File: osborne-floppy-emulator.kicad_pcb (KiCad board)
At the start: 2 copper layers, 76.2 x 94 mm, 67 parts, among them J1 Connector Out, J2 USB_A, J3 SWD Connector, J4 Connector In, Q1 BC557, Q2 BC547, Q3 T2N7002BK, Q4 BC547, Q5 BC547, Q6 BC547, Q7 BC547, Q8 BC547, Q9 BC547, U1 W25Q16JVSSIM, U2 RP2040, U3 TL494

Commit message: fixed issue with OCP comparator polarity
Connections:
- R13 pad 2: Net-(U3-2IN+) -> Net-(U3-2IN-)
- R9 pad 1: Net-(U3-2IN+) -> Net-(U3-2IN-)
- U3 pad 15: GND -> Net-(U3-2IN-)
- U3 pad 16: Net-(U3-2IN+) -> GND
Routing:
- net Net-(U3-2IN-): track 0.00 -> 66.5 mm
- net GND: track 107.9 -> 41.4 mm
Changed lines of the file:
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@@
 	(net 59 "Net-(R12-Pad1)")
 	(net 60 "Net-(U3-1IN+)")
-	(net 61 "Net-(U3-2IN+)")
+	(net 61 "Net-(U3-2IN-)")
 	(net 62 "Net-(U3-RT)")
 	(net 63 "/Processor/Chip D+")
@@
 			)
 		)
-		(property "Mouser part no." " 603-MFR-25FTE52-7K5"
+		(property "Mouser part no." " 603-MFR-12FTF52-7K5"
 			(at 0 0 30)
 			(unlocked yes)
@@
 			)
 		)
-		(property "Mouser part no." " 603-MFR-25FTE52-27K"
+		(property "Mouser part no." " 603-MFR-12FTF52-27K"
 			(at 0 0 -135)
 			(unlocked yes)
@@
 			)
 		)
-		(property "Mouser part no." " 603-MFR-25FTE52-3K6 "
+		(property "Mouser part no." " 603-MFR-12FTF52-3K6 "
 			(at 0 0 -75)
 			(unlocked yes)
@@
 			)
 		)
-		(property "Mouser part no." " 603-MFR-25FTE52-27K"
+		(property "Mouser part no." " 603-MFR-12FTF52-27K"
 			(at 0 0 -120)
 			(unlocked yes)
@@
 			)
 		)
-		(property "Mouser part no." " 737-PH2-18-UA"
+		(property "Mouser part no." " 649-67996-434HLF"
 			(at 0 0 0)
 			(unlocked yes)
@@
 			)
 		)
-		(property "Mouser part no." " 603-MFR-25FTE52-27K"
+		(property "Mouser part no." " 603-MFR-12FTF52-27K"
 			(at 0 0 180)
 			(unlocked yes)
@@
 			)
 		)
-		(property "Mouser part no." " 603-MFR-25FTE52-27K"
+		(property "Mouser part no." " 603-MFR-12FTF52-27K"
 			(at 0 0 0)
 			(unlocked yes)
@@
 			(layers "*.Cu" "*.Mask")
 			(remove_unused_layers no)
-			(net 5 "GND")
+			(net 61 "Net-(U3-2IN-)")
 			(pinfunction "2IN-")
 			(pintype "input")
@@
 			(layers "*.Cu" "*.Mask")
 			(remove_unused_layers no)
-			(net 61 "Net-(U3-2IN+)")
+			(net 5 "GND")
 			(pinfunction "2IN+")
 			(pintype "input")
@@
 			)
 		)
-		(property "Mouser part no." " 737-RS2-20-G"
+		(property "Mouser part no." " 710-61304021821"
 			(at 0 0 180)
 			(unlocked yes)
@@
 			)
 		)
-		(property "Mouser part no." " 603-MFR-25FTE52-56R"
+		(property "Mouser part no." " 603-MFR-12FTF52-56R"
 			(at 0 0 180)
 			(unlocked yes)
@@
 			(layers "*.Cu" "*.Mask")
 			(remove_unused_layers no)
-			(net 61 "Net-(U3-2IN+)")
+			(net 61 "Net-(U3-2IN-)")
 			(pintype "passive")
 		)
@@
 			)
 		)
-		(property "Mouser part no." " 603-MFR-25FTE52-27K"
+		(property "Mouser part no." " 603-MFR-12FTF52-27K"
 			(at 0 0 165)
 			(unlocked yes)
@@
 			)
 		)
-		(property "Mouser part no." " 603-MFR-25FTE52-27K"
+		(property "Mouser part no." " 603-MFR-12FTF52-27K"
 			(at 0 0 165)
 			(unlocked yes)
@@
 			)
 		)
-		(property "Mouser part no." " 603-MFR-25FTE52-27K"
+		(property "Mouser part no." " 603-MFR-12FTF52-27K"
 			(at 0 0 180)
 			(unlocked yes)
@@
 			)
 		)
-		(property "Mouser part no." " 603-MFR-25FTE52-12K"
+		(property "Mouser part no." " 603-MFR-12FTF52-12K"
 			(at 0 0 150)
 			(unlocked yes)
@@
 			)
 		)
-		(property "Mouser part no." " 603-MFR-25FTE52-27K"
+		(property "Mouser part no." " 603-MFR-12FTF52-27K"
 			(at 0 0 150)
 			(unlocked yes)
@@
 			)
 		)
-		(property "Mouser part no." " 603-MFR-25FTE52-27K"
+		(property "Mouser part no." " 603-MFR-12FTF52-27K"
 			(at 0 0 180)
 			(unlocked yes)
@@
 			)
 		)
-		(property "Mouser part no." " 603-MFR-25FTE52-27K"
+		(property "Mouser part no." " 603-MFR-12FTF52-27K"
 			(at 0 0 90)
 			(unlocked yes)
@@
 			(layers "*.Cu" "*.Mask")
 			(remove_unused_layers no)
-			(net 61 "Net-(U3-2IN+)")
+			(net 61 "Net-(U3-2IN-)")
 			(pintype "passive")
 		)
@@
 	)
 	(segment
-		(start 153.6 38.8)
-		(end 155 37.2)
-		(width 0.6)
-		(layer "F.Cu")
-		(net 5)
-	)
-	(segment
 		(start 150.2 85.6)
 		(end 149.2 86.2)
@@
 	)
 	(segment
-		(start 155.4 34.8)
-		(end 155.4 25)
-		(width 0.6)
-		(layer "F.Cu")
-		(net 5)
-	)
-	(segment
 		(start 151.8 88.0625)
 		(end 151.2 89.6)
@@
 	)
 	(segment
-		(start 151.599999 39.000001)
-		(end 153.6 38.8)
-		(width 0.6)
-		(layer "F.Cu")
-		(net 5)
-	)
-	(segment
-		(start 155.4 25)
-		(end 153.6 19.6)
-		(width 0.6)
-		(layer "F.Cu")
-		(net 5)
-	)
-	(segment
 		(start 143.2 91.6)
 		(end 142.4 92.8)
@@
 	)
 	(segment
-		(start 148.2 16.4)
-		(end 112.6 16.4)
-		(width 0.6)
-		(layer "F.Cu")
-		(net 5)
-	)
-	(segment
 		(start 124.700001 40.599999)
 		(end 124.6 43)
@@
 	)
 	(segment
-		(start 149.02 38.96)
-		(end 151.599999 39.000001)
-		(width 0.6)
-		(layer "F.Cu")
-		(net 5)
-	)
-	(segment
 		(start 116.6 38.499999)
 		(end 118.2 35.2)
@@
 	)
 	(segment
-		(start 153.6 19.6)
-		(end 148.2 16.4)
-		(width 0.6)
-		(layer "F.Cu")
-		(net 5)
-	)
-	(segment
 		(start 151.2 85)
 		(end 150.2 85.6)
@@
 	)
 	(segment
-		(start 155 37.2)
-		(end 155.4 34.8)
-		(width 0.6)
-		(layer "F.Cu")
-		(net 5)
-	)
-	(segment
 		(start 159.466222 82.046462)
 		(end 160.8 82.4)
@@
 	)
 	(segment
+		(start 153.6 38.8)
+		(end 155 37.2)
+		(width 0.6)
+		(layer "F.Cu")
+		(net 61)
+	)
+	(segment
+		(start 155.4 34.8)
+		(end 155.4 25)
+		(width 0.6)
+		(layer "F.Cu")
+		(net 61)
+	)
+	(segment
+		(start 151.599999 39.000001)
+		(end 153.6 38.8)
+		(width 0.6)
+		(layer "F.Cu")
+		(net 61)
+	)
+	(segment
+		(start 155.4 25)
+		(end 153.6 19.6)
+		(width 0.6)
+		(layer "F.Cu")
+		(net 61)
+	)
+	(segment
+		(start 148.2 16.4)
+		(end 112.6 16.4)
+		(width 0.6)
+		(layer "F.Cu")
+		(net 61)
+	)
+	(segment
+		(start 149.02 38.96)
+		(end 151.599999 39.000001)
+		(width 0.6)
+		(layer "F.Cu")
+		(net 61)
+	)
+	(segment
+		(start 153.6 19.6)
+		(end 148.2 16.4)
+		(width 0.6)
+		(layer "F.Cu")
+		(net 61)
+	)
+	(segment
+		(start 155 37.2)
+		(end 155.4 34.8)
+		(width 0.6)
+		(layer "F.Cu")
+		(net 61)
+	)
+	(segment

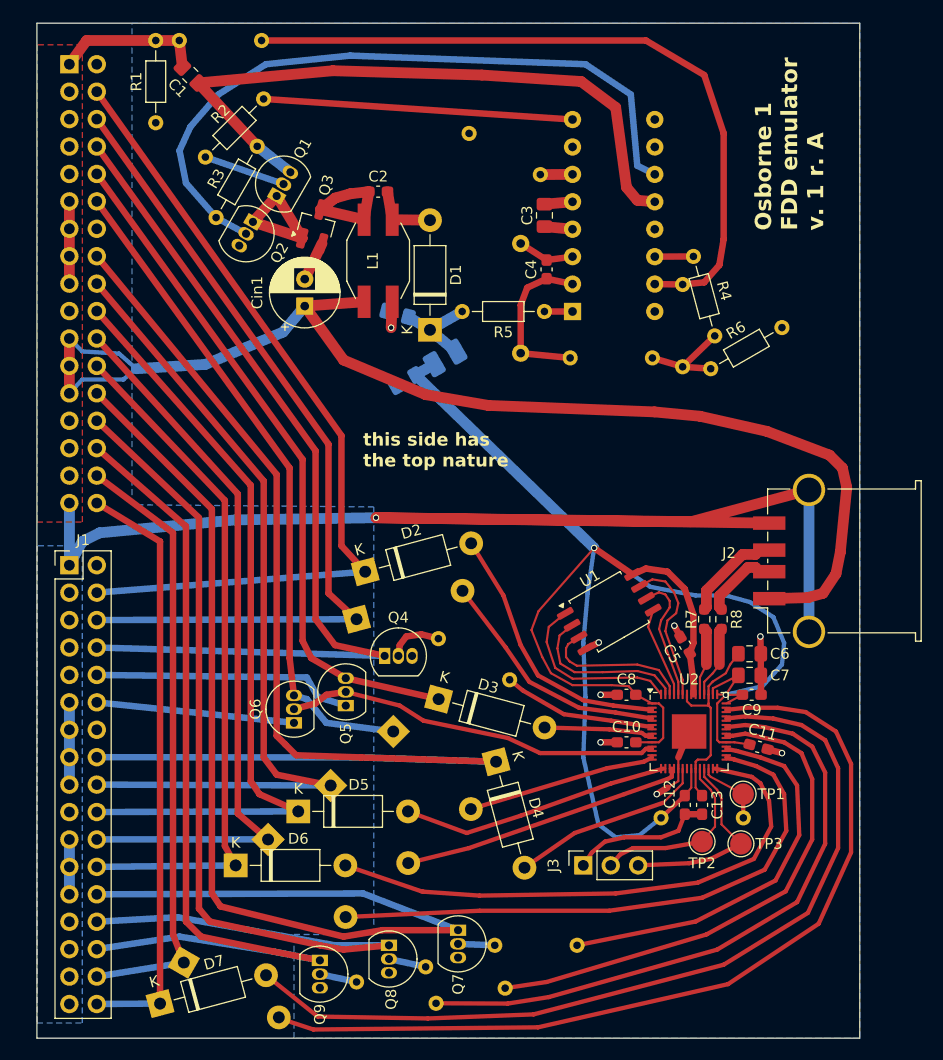
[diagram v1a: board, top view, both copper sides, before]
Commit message: Change a whole bunch of stuff for v2
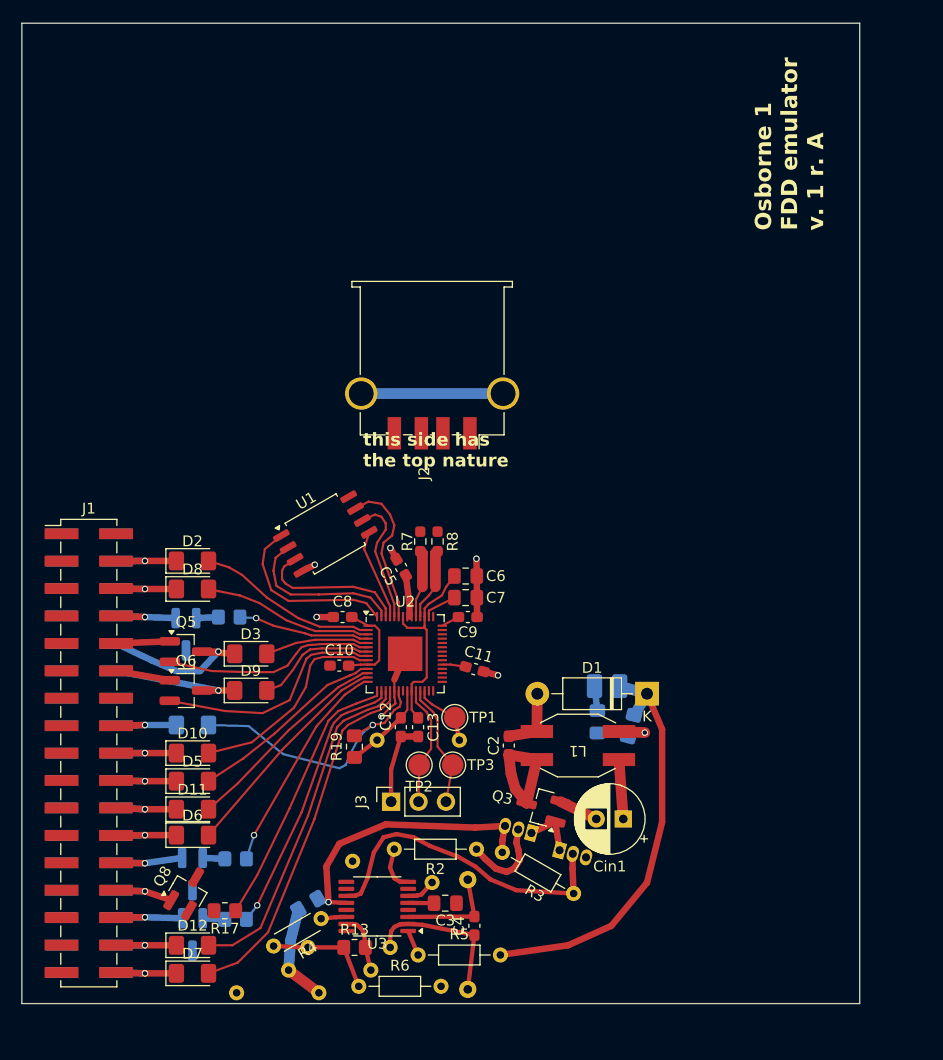
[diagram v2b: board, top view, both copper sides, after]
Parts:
- added R19: 27k, Resistor_SMD:R_0805_2012Metric_Pad1.20x1.40mm_HandSolder, F.Cu at (121.2, 81.8)
- C1, Q1, Q2, R1: moved to B.Cu
- D10, D11, D12, D8, D9: value 1N4004 -> FDLL4148; footprint Diode_THT:D_DO-41_SOD81_P10.16mm_Horizontal -> Diode_SMD:D_1206_3216Metric_Pad1.42x1.75mm_HandSolder; moved to F.Cu
- D2, D3, D5, D6, D7: value 1N4004 -> FDLL4148; footprint Diode_THT:D_DO-41_SOD81_P10.16mm_Horizontal -> Diode_SMD:D_1206_3216Metric_Pad1.42x1.75mm_HandSolder
- D4: value 1N4004 -> FDLL4148; footprint Diode_THT:D_DO-41_SOD81_P10.16mm_Horizontal -> Diode_SMD:D_1206_3216Metric_Pad1.42x1.75mm_HandSolder; moved to B.Cu
- J1: footprint Connector_PinHeader_2.54mm:PinHeader_2x17_P2.54mm_Vertical -> Connector_PinHeader_2.54mm:PinHeader_2x17_P2.54mm_Vertical_SMD
- J4: footprint Connector_PinSocket_2.54mm:PinSocket_2x17_P2.54mm_Vertical -> Connector_PinSocket_2.54mm:PinSocket_2x17_P2.54mm_Vertical_SMD
- Q4, Q7, Q9: value BC547 -> BC847C; footprint Package_TO_SOT_THT:TO-92_Inline -> Package_TO_SOT_SMD:SOT-23_Handsoldering; moved to B.Cu
- Q5, Q6, Q8: value BC547 -> BC847C; footprint Package_TO_SOT_THT:TO-92_Inline -> Package_TO_SOT_SMD:SOT-23_Handsoldering
- R13, R17: footprint Resistor_THT:R_Axial_DIN0204_L3.6mm_D1.6mm_P7.62mm_Horizontal -> Resistor_SMD:R_0805_2012Metric_Pad1.20x1.40mm_HandSolder; moved to F.Cu
- R14, R16, R18: footprint Resistor_THT:R_Axial_DIN0204_L3.6mm_D1.6mm_P7.62mm_Horizontal -> Resistor_SMD:R_0805_2012Metric_Pad1.20x1.40mm_HandSolder
- R4: footprint Resistor_THT:R_Axial_DIN0204_L3.6mm_D1.6mm_P7.62mm_Horizontal -> Resistor_THT:R_Axial_DIN0204_L3.6mm_D1.6mm_P5.08mm_Horizontal
- U3: footprint Package_DIP:DIP-16_W7.62mm_Socket -> Package_SO:TSSOP-16_4.4x5mm_P0.65mm; moved to F.Cu
- moved R1 89.5 mm to (117.9, 104.6), turned to 180 degrees
- moved R9 86.7 mm to (122.7, 102.5)
- moved C1 77.6 mm to (116.9, 96.4), turned to -150 degrees
- moved R2 70.5 mm to (124.9, 91.3), turned to 0 degrees
- moved R4 70.4 mm to (118.1, 97.7), turned to -150 degrees
- moved R3 69.2 mm to (134.9, 91.6), turned to -30 degrees
- moved R10 66.3 mm to (128.4, 94.4), turned to 165 degrees
- moved R6 65.8 mm to (121.6, 104.0), turned to 0 degrees
- moved Q2 64.8 mm to (140.2, 91.4), turned to -15 degrees
- moved C3 64.4 mm to (129.6, 96.3), turned to 0 degrees
- moved J4 63.8 mm to (96.6, 82.4)
- moved Q1 63.5 mm to (137.6, 89.8), turned to 165 degrees
- moved R12 63.2 mm to (116.9, 100.4), turned to 0 degrees
- moved R13 61.8 mm to (121.2, 100.4), turned to 0 degrees
- moved C4 61.2 mm to (132.3, 98.4)
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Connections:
- Q5 pad 2: /Connector/FDD Enable -> /Connector/DS 1 Enable
- Q6 pad 2: /Connector/FDD Enable -> /Connector/DS 2 Enable
- U2 pad 11: /Connector/FDD Enable -> /Level Shifter/~{Step} CMOS
- U2 pad 12: /Connector/FDD Enable -> /Level Shifter/~{Write Data} CMOS
- U2 pad 13: /Level Shifter/~{DS 2} CMOS -> /Level Shifter/~{Write Gate} CMOS
- U2 pad 14: /Level Shifter/~{DS 2} CMOS -> /Level Shifter/Track 00 CMOS
- U2 pad 15: /Level Shifter/~{Step} CMOS -> /Level Shifter/Write Protect CMOS
- U2 pad 16: /Level Shifter/~{Step} CMOS -> /Level Shifter/~{Read Data} CMOS
- U2 pad 17: /Level Shifter/~{Direction} CMOS -> /Level Shifter/~{Side Select} CMOS
- U2 pad 18: /Level Shifter/~{Direction} CMOS -> /Level Shifter/~{Late} CMOS
- U2 pad 27: /Level Shifter/~{Write Gate} CMOS -> Net-(U2-GPIO16)
- U2 pad 28: /Level Shifter/~{Write Gate} CMOS -> Net-(U2-GPIO17)
- U2 pad 29: /Level Shifter/~{Write Data} CMOS -> Net-(U2-GPIO18)
- U2 pad 3: /Level Shifter/~{TG43} CMOS -> /Level Shifter/~{Early} CMOS
- U2 pad 30: /Level Shifter/~{Write Data} CMOS -> Net-(U2-GPIO19)
- U2 pad 31: /Level Shifter/Track 00 CMOS -> Net-(U2-GPIO20)
- U2 pad 32: /Level Shifter/Track 00 CMOS -> Net-(U2-GPIO21)
- U2 pad 34: /Level Shifter/Write Protect CMOS -> Net-(U2-GPIO22)
- U2 pad 35: /Level Shifter/Write Protect CMOS -> Net-(U2-GPIO23)
- U2 pad 36: /Level Shifter/~{Read Data} CMOS -> Net-(U2-GPIO24)
- U2 pad 37: /Level Shifter/~{Read Data} CMOS -> Net-(U2-GPIO25)
- U2 pad 38: /Level Shifter/~{Late} CMOS -> Net-(U2-GPIO26_ADC0)
- U2 pad 39: /Level Shifter/~{Late} CMOS -> Net-(U2-GPIO27_ADC1)
- U2 pad 4: /Level Shifter/~{Early} CMOS -> /Level Shifter/Index CMOS
- U2 pad 40: /Level Shifter/~{Side Select} CMOS -> Net-(U2-GPIO28_ADC2)
- U2 pad 41: /Level Shifter/~{Side Select} CMOS -> Net-(U2-GPIO29_ADC3)
- U2 pad 5: /Level Shifter/~{Early} CMOS -> /Level Shifter/~{DS 1} CMOS
- U2 pad 6: /Level Shifter/Index CMOS -> /Connector/DS 1 Enable
- U2 pad 7: /Level Shifter/Index CMOS -> /Level Shifter/~{DS 2} CMOS
- U2 pad 8: /Level Shifter/~{DS 1} CMOS -> /Connector/DS 2 Enable
- U2 pad 9: /Level Shifter/~{DS 1} CMOS -> /Level Shifter/~{Direction} CMOS
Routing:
- net +3V3: track 160.8 -> 30.7 mm, vias 2 -> 0
- net /Connector/-0V: track 139.6 -> 22.3 mm, vias 1 -> 0
- net +5V: track 118.7 -> 5.51 mm
- net /Connector/~{4MHz}: track 108.5 -> 8.27 mm, vias 0 -> 1
- net /Connector/~{Track 00}: track 108.6 -> 8.84 mm, vias 0 -> 1
- net /Connector/~{Write Protect}: track 95.0 -> 7.92 mm, vias 0 -> 1
- net /Connector/~{Index}: track 84.7 -> 8.21 mm, vias 0 -> 1
- net /Connector/Read Data: track 81.7 -> 8.81 mm, vias 0 -> 1
- net /Connector/~{Early}: track 78.4 -> 8.27 mm, vias 0 -> 1
- net /Connector/~{Direction}: track 78.3 -> 8.27 mm, vias 0 -> 1
- net /Connector/~{TG43}: track 77.5 -> 8.27 mm, vias 0 -> 1
- net /Connector/~{Step}: track 73.0 -> 8.27 mm, vias 0 -> 1
- net Net-(U3-2IN-): track 66.5 -> 5.50 mm
- net /Connector/~{Write Data}: track 68.6 -> 8.27 mm, vias 0 -> 1
- net /Connector/~{Write Gate}: track 64.1 -> 8.27 mm, vias 0 -> 1
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- removed copper zone on B.Cu, net /Connector/-0V
- removed copper zone on F.Cu, net /Connector/-0V
- removed copper zone on B.Cu, net GND
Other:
- board size 76.2 x 94 mm -> 77.6 x 90.8 mm
